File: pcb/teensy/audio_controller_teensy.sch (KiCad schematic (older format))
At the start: 2 parts

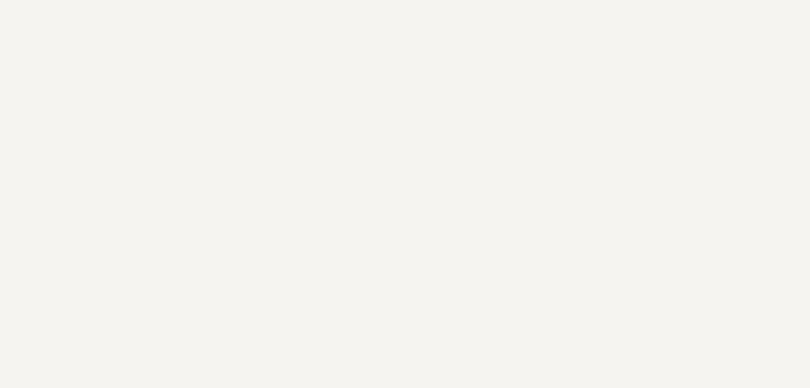
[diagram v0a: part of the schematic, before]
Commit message: Progress towards schematic v1.0.
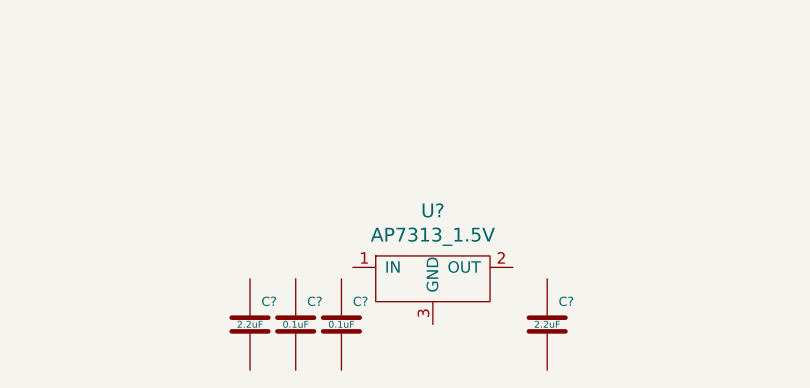
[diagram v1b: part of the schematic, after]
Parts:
- added C? (x2): 2.2uF, footprints:SM1210, symbol 2.2uF
- added C? (x2): 0.1uF, footprints:SM1210, symbol 0.1uF
- added U?: AP7313_1.5V, footprints:SOT-23-3, symbol AP7313_1.5V
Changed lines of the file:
@@
+	1    0    0    -1
+$EndComp
+$Comp
+L AP7313_1.5V U?
+U 1 1 57C8ABBD
+P 2400 3600
+F 0 "U?" H 2400 3847 60  0000 C CNN
+F 1 "AP7313_1.5V" H 2400 3741 60  0000 C CNN
+F 2 "footprints:SOT-23-3" H 2450 3300 60  0001 C CNN
+F 3 "" H 2400 3600 60  0001 C CNN
+F 4 "digikey" H 2650 3500 60  0001 C CNN "Vendor"
+F 5 "AP7313-15SAG-7DICT-ND" H 2750 3600 60  0001 C CNN "PartNumber"
+F 6 "Linear Voltage Regulator IC Positive Fixed 1 Output 1.5V 150mA SOT-23-3" H 2850 3700 60  0001 C CNN "Description"
+	1    2400 3600
+	1    0    0    -1
+$EndComp
+$Comp
+L 2.2uF C?
+U 1 1 57C8D133
+P 1600 3850
+F 0 "C?" H 1650 3950 40  0000 L CNN
+F 1 "2.2uF" H 1600 3850 30  0000 C CNN
+F 2 "footprints:SM1210" H 1638 3700 30  0001 C CNN
+F 3 "" H 1600 3850 60  0000 C CNN
+F 4 "digikey" H 1700 4050 60  0001 C CNN "Vendor"
+F 5 "478-3591-1-ND" H 1800 4150 60  0001 C CNN "PartNumber"
+F 6 "2.2uF 50V Ceramic Capacitor X7R 1210" H 1900 4250 60  0001 C CNN "Description"
+	1    1600 3850
+	1    0    0    -1
+$EndComp
+$Comp
+L 0.1uF C?
+U 1 1 57C8D1F2
+P 1800 3850
+F 0 "C?" H 1850 3950 40  0000 L CNN
+F 1 "0.1uF" H 1800 3850 30  0000 C CNN
+F 2 "footprints:SM1210" H 1838 3700 30  0001 C CNN
+F 3 "" H 1800 3850 60  0000 C CNN
+F 4 "digikey" H 1900 4050 60  0001 C CNN "Vendor"
+F 5 "478-3586-1-ND" H 2000 4150 60  0001 C CNN "PartNumber"
+F 6 "CAP CER 0.1UF 50V 10% X7R 1210" H 2100 4250 60  0001 C CNN "Description"
+	1    1800 3850
+	1    0    0    -1
+$EndComp
+$Comp
+L 0.1uF C?
+U 1 1 57C8D519
+P 2000 3850
+F 0 "C?" H 2050 3950 40  0000 L CNN
+F 1 "0.1uF" H 2000 3850 30  0000 C CNN
+F 2 "footprints:SM1210" H 2038 3700 30  0001 C CNN
+F 3 "" H 2000 3850 60  0000 C CNN
+F 4 "digikey" H 2100 4050 60  0001 C CNN "Vendor"
+F 5 "478-3586-1-ND" H 2200 4150 60  0001 C CNN "PartNumber"
+F 6 "CAP CER 0.1UF 50V 10% X7R 1210" H 2300 4250 60  0001 C CNN "Description"
+	1    2000 3850
+	1    0    0    -1
+$EndComp
+$Comp
+L 2.2uF C?
+U 1 1 57C8D5F7
+P 2900 3850
+F 0 "C?" H 2950 3950 40  0000 L CNN
+F 1 "2.2uF" H 2900 3850 30  0000 C CNN
+F 2 "footprints:SM1210" H 2938 3700 30  0001 C CNN
+F 3 "" H 2900 3850 60  0000 C CNN
+F 4 "digikey" H 3000 4050 60  0001 C CNN "Vendor"
+F 5 "478-3591-1-ND" H 3100 4150 60  0001 C CNN "PartNumber"
+F 6 "2.2uF 50V Ceramic Capacitor X7R 1210" H 3200 4250 60  0001 C CNN "Description"
+	1    2900 3850
 	1    0    0    -1
 $EndComp
